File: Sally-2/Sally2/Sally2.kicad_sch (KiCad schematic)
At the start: 34 parts, among them J1 Power SW, J10 GND +5V, J11 A16, J2 Power LED, J3 USB_B, J4 PowerUSB, J5 GND +5V, J6 Barrel_Jack, J7 GND +5V, J8 PowerBarrel, J9 + A14 -, SW1 Reset, U1 GAL16V8 - IO decoder, U2 Z80ACPU, U3 GAL16V8 - ADR decoder, U4 27C256, U5 628128_DIP32_SSOP32, U6 GAL16V8 - glue logic, U7 74LS259, X1 16Mhz

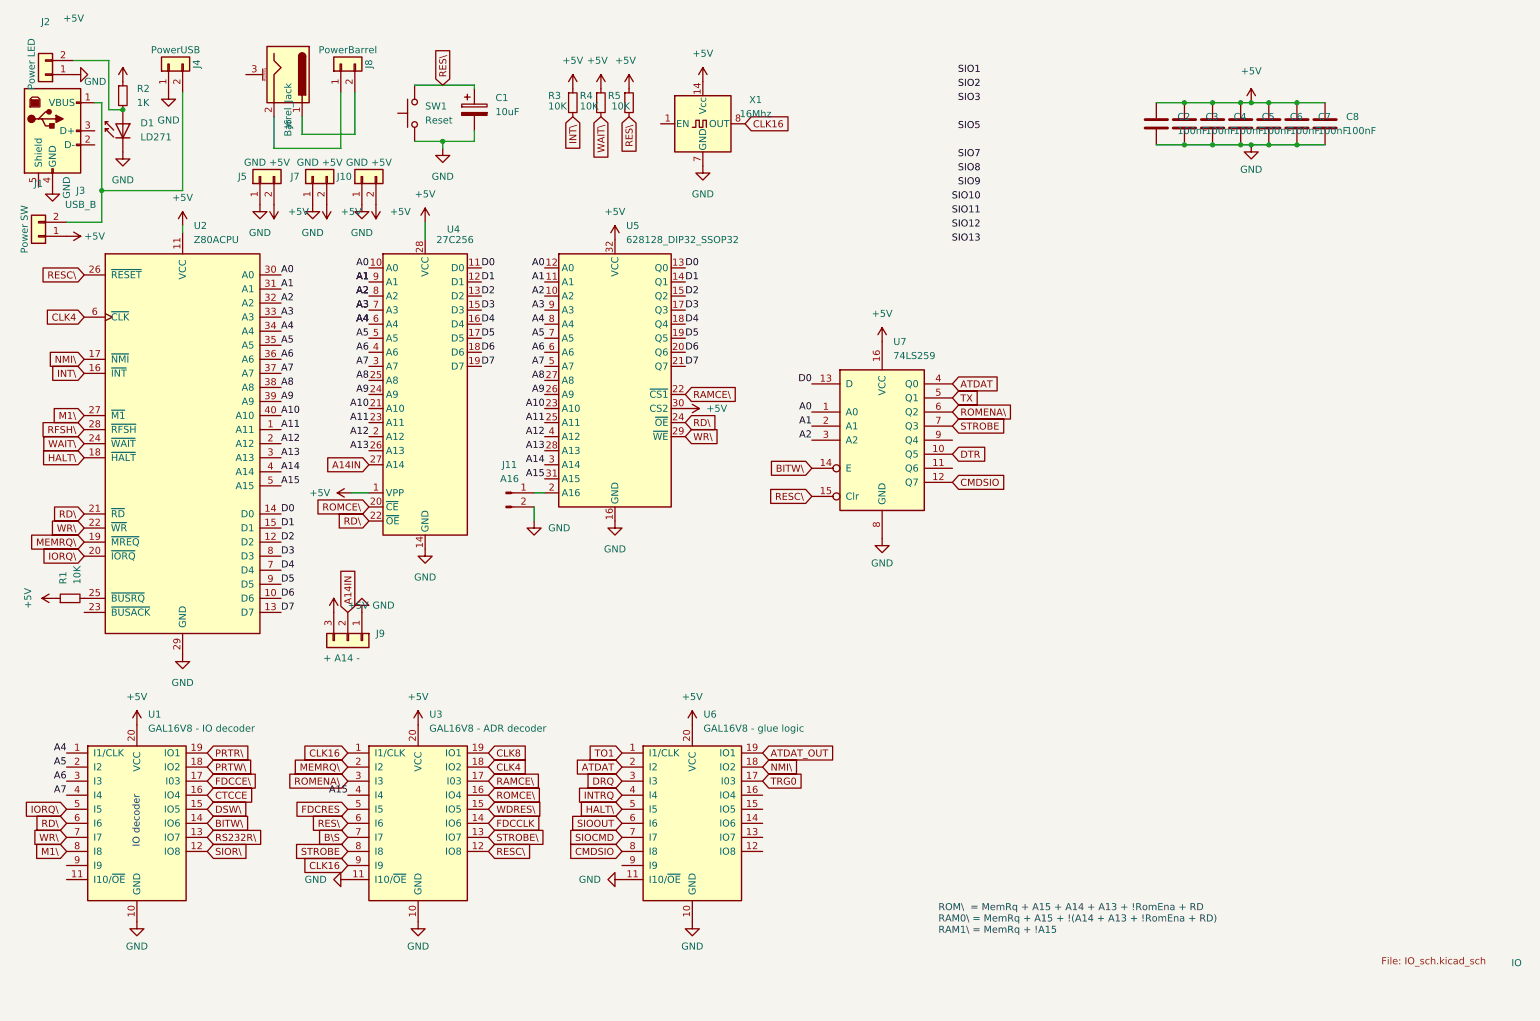
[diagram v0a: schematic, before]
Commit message: workover part 1
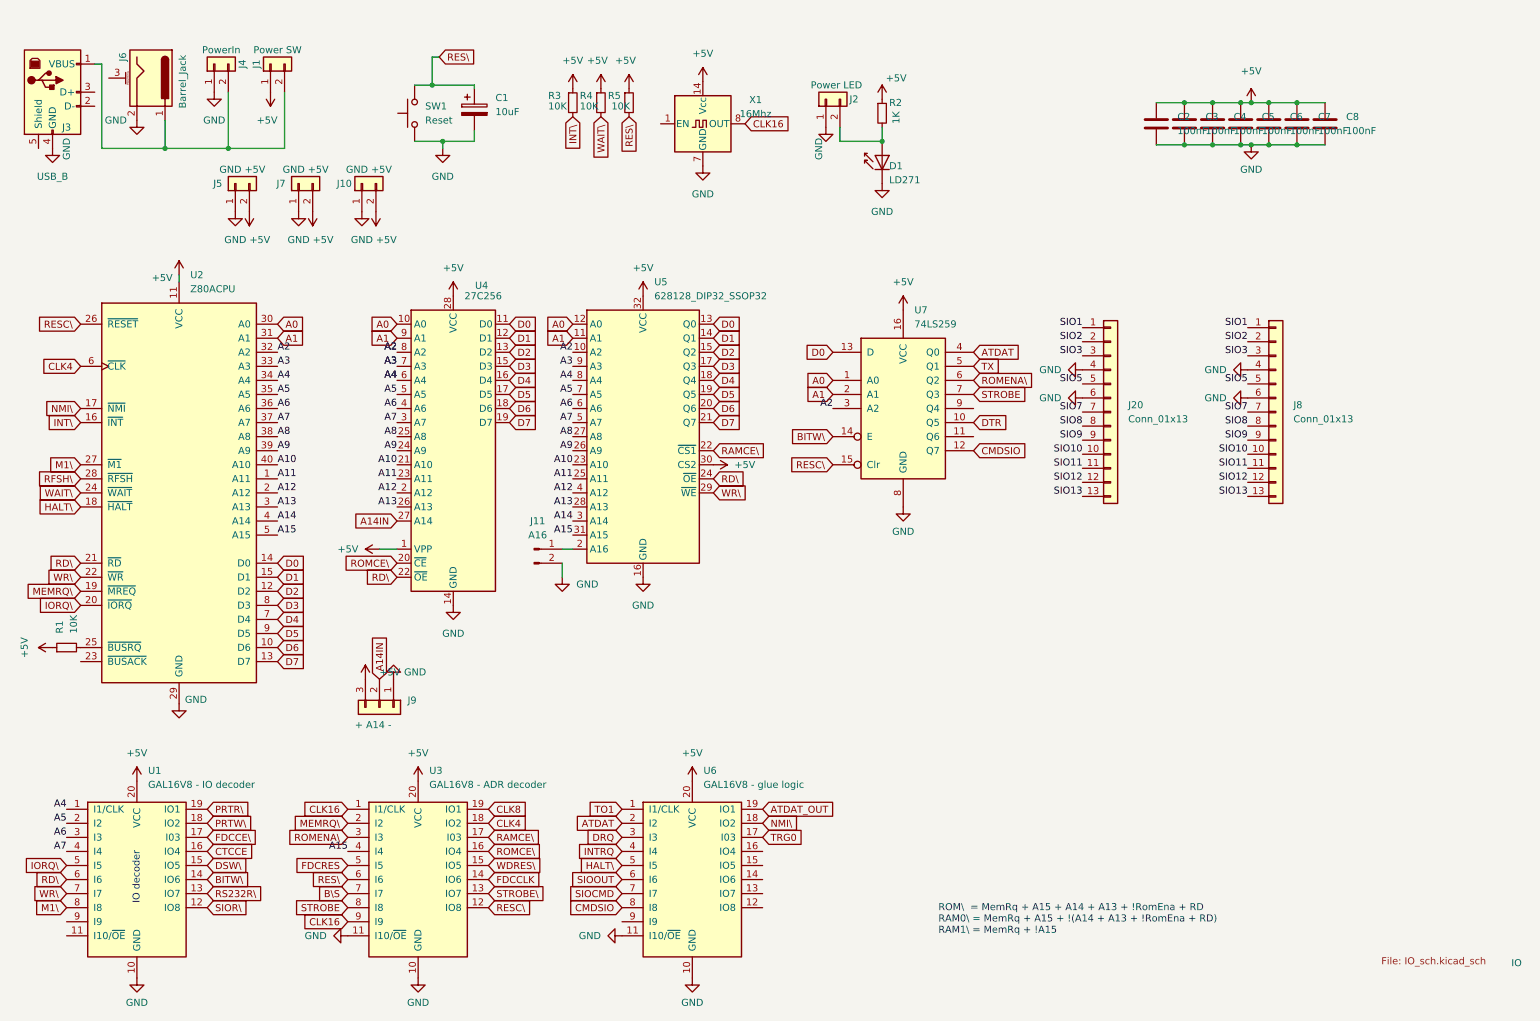
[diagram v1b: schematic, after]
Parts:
- removed J8: PowerBarrel, Connector_PinHeader_2.54mm:PinHeader_1x02_P2.54mm_Vertical, symbol Connector_Generic:Conn_01x02
- added J20, J8: Conn_01x13, Sally2:SIO_JACK, symbol Connector_Generic:Conn_01x13
- J4: value PowerUSB -> PowerIn
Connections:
- net GND: now also J6.2, J20.4 (Pin_4), J20.6 (Pin_6), J8.4 (Pin_4), J8.6 (Pin_6)
- net SIO1: now also J20.1 (Pin_1), J8.1 (Pin_1)
- net SIO10: now also J20.10 (Pin_10), J8.10 (Pin_10)
- net SIO11: now also J20.11 (Pin_11), J8.11 (Pin_11)
- net SIO12: now also J20.12 (Pin_12), J8.12 (Pin_12)
- net SIO13: now also J20.13 (Pin_13), J8.13 (Pin_13)
- net SIO2: now also J20.2 (Pin_2), J8.2 (Pin_2)
- net SIO3: now also J20.3 (Pin_3), J8.3 (Pin_3)
- net SIO5: now also J20.5 (Pin_5), J8.5 (Pin_5)
- net SIO7: now also J20.7 (Pin_7), J8.7 (Pin_7)
- net SIO8: now also J20.8 (Pin_8), J8.8 (Pin_8)
- net SIO9: now also J20.9 (Pin_9), J8.9 (Pin_9)
- net at J6.1: now also J1.2 (Pin_2), J3.1 (VBUS), J4.2 (Pin_2)
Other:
- moved on the sheet: D1, J1, J10, J11, J2, J3, J4, J5, J6, J7, J9, R1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
